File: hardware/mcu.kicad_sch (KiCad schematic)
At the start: 61 parts, among them J1 TYPE-C 16PIN 2MD(073), J2 Conn_ARM_JTAG_SWD_10, J22 Conn_01x16, J3 Conn_02x03_Odd_Even, J4 Conn_02x04_Odd_Even, Q1 DMP1045U-7, Q4 SS8050, Q5 SL1254-3, SW1 MK-12C01-G1.5, SW2 TS-1095PS-A1B2-C3D2, SW3 TS-1095PS-A1B2-C3D2, SW4 10*10*9-6P WX, U1 TPS63031DSK, U10 PY25Q128HA, U2 RP2350A-QFN60, U7 24CS02, Y1 12Mhz

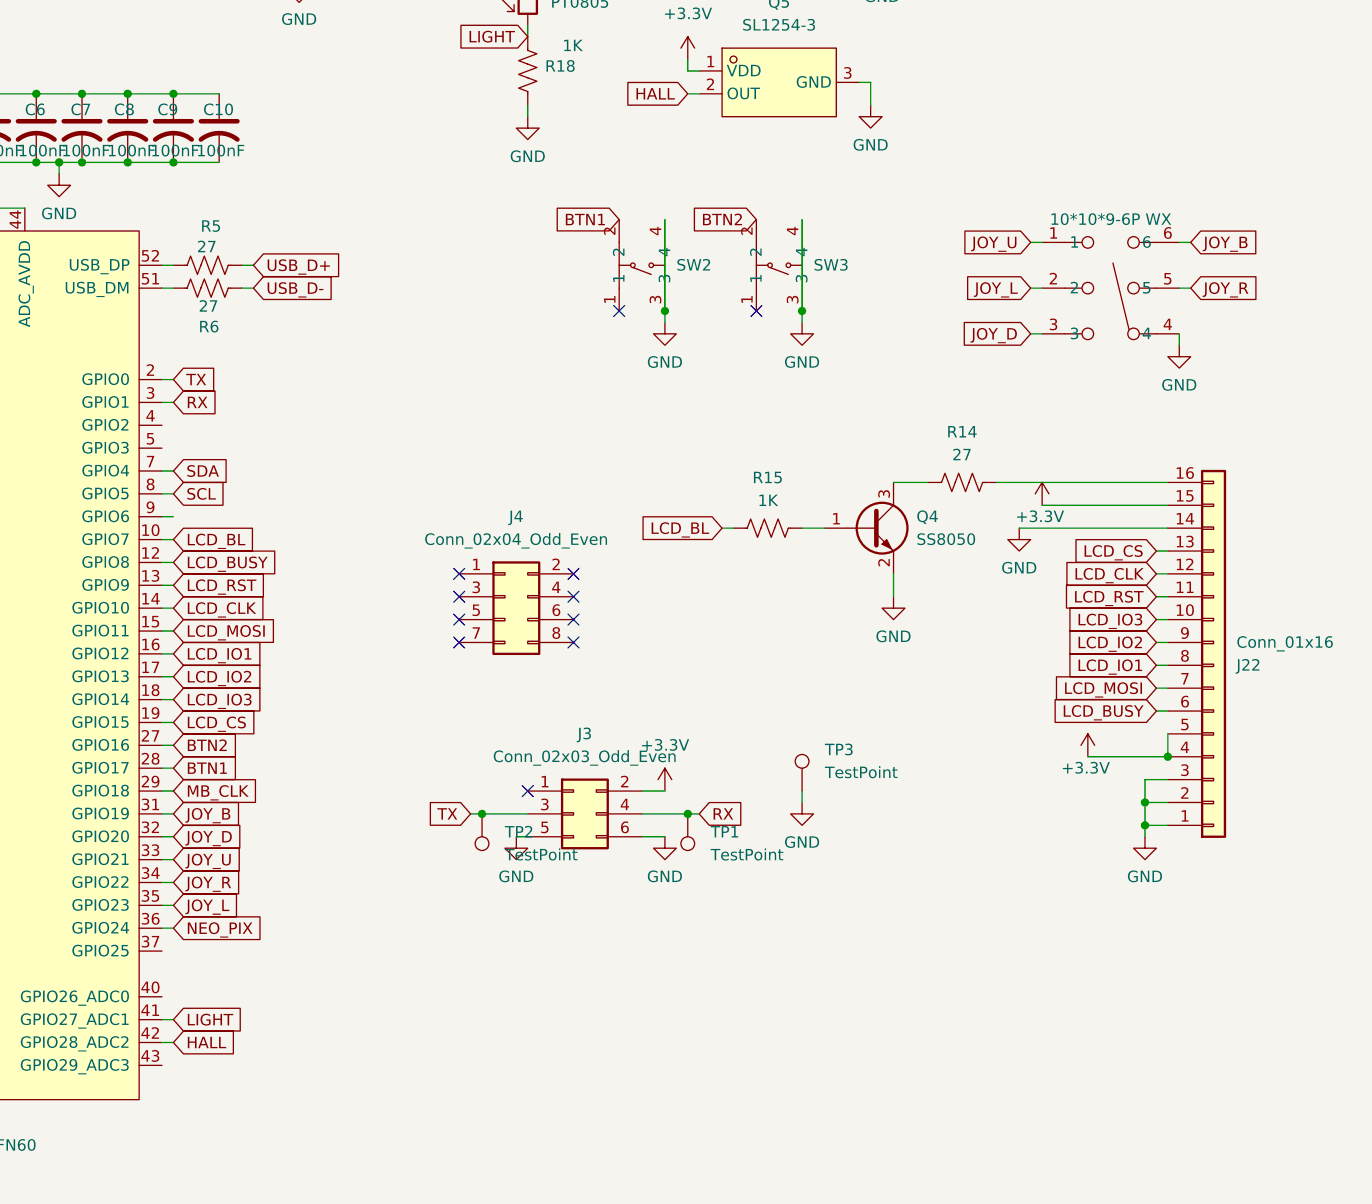
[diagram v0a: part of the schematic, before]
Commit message: prototype v0.3
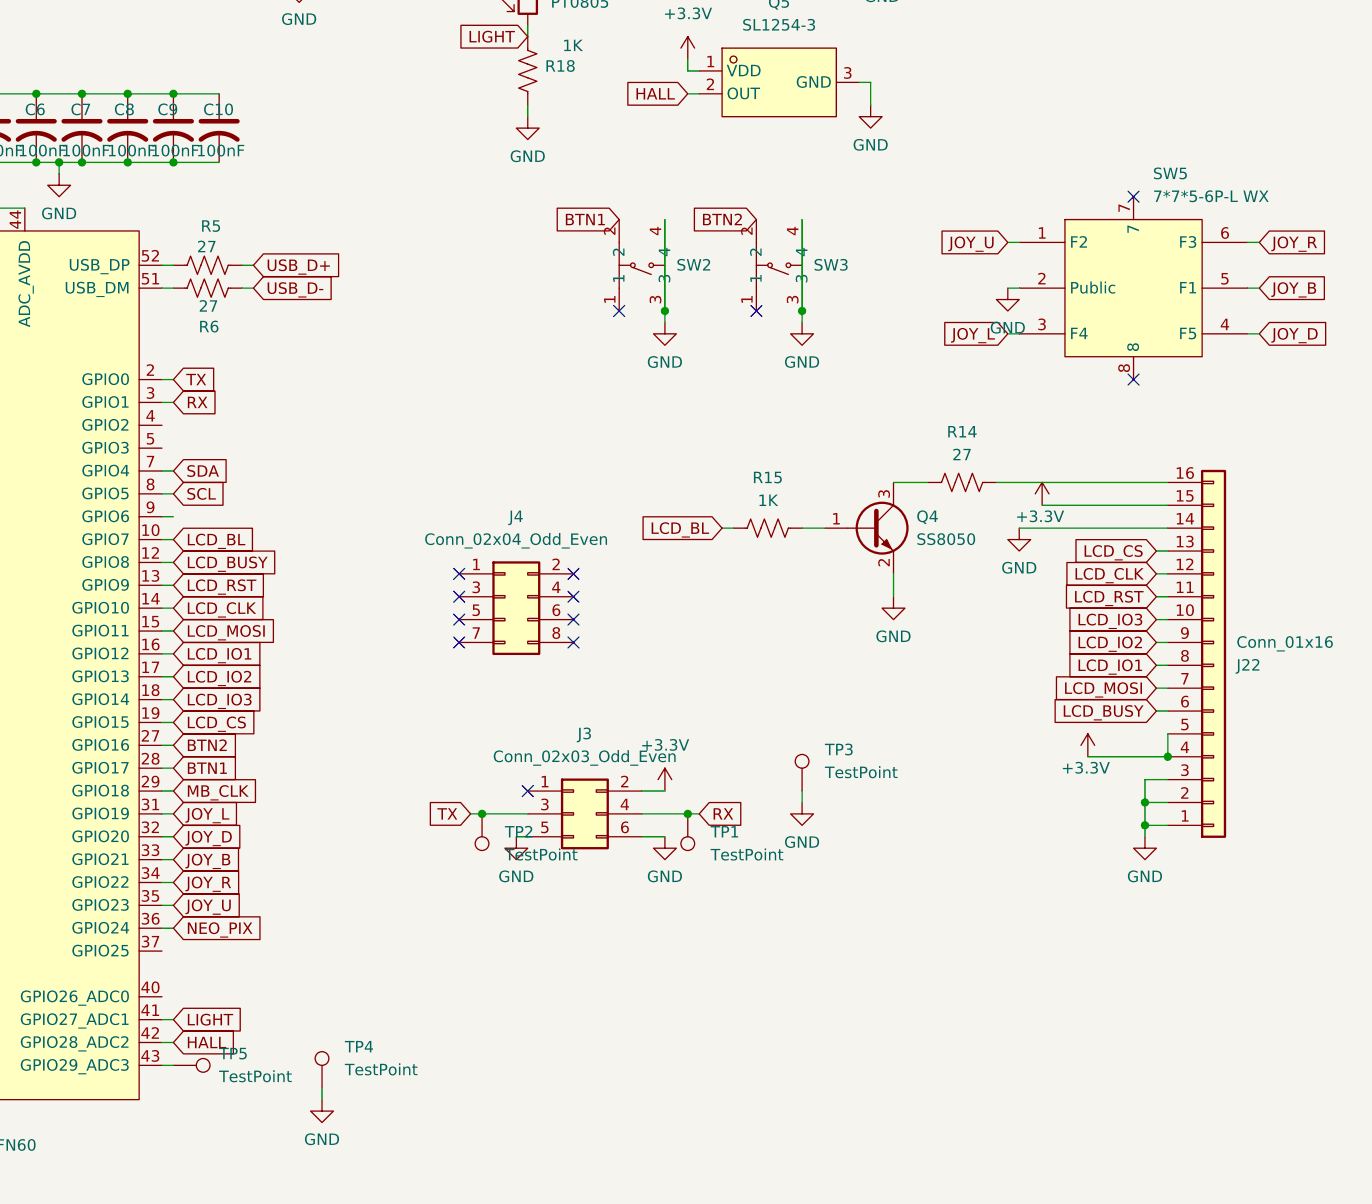
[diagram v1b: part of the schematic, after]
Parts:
- removed SW4: 10*10*9-6P WX, easyeda2kicad:SW-SMD-6P-L10.5-W10.0_C2858290, symbol easyeda2kicad:10*10*9-6PWX
- added SW5: 7*7*5-6P-L WX, easyeda2kicad:SW-SMD_8P-L7.0-W7.0-P1.40-LS7.4-TL, symbol easyeda2kicad:7*7*5-6P-LWX
- added TP4, TP5: TestPoint, TestPoint:TestPoint_Pad_D1.0mm, symbol Connector:TestPoint
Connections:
- net GND: now also SW5.2 (Public), TP4.1
- net JOY_B: now also U2.33 (GPIO21), SW5.5 (F1); no longer U2.31 (GPIO19)
- net JOY_D: now also SW5.4 (F5)
- net JOY_L: now also U2.31 (GPIO19), SW5.3 (F4); no longer U2.35 (GPIO23)
- net JOY_R: now also SW5.6 (F3)
- net JOY_U: now also U2.35 (GPIO23), SW5.1 (F2); no longer U2.33 (GPIO21)
- net at U2.43 (GPIO29_ADC3): now also TP5.1
- no-connect marks 15 -> 17
